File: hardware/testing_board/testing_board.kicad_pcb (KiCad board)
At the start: 2 copper layers, 100.6 x 99.1 mm, 75 parts, among them J1 Conn_01x04, J16 Conn_01x04, J2 Conn_01x04, J3 Conn_01x04, J4 Conn_01x04, J5 Conn_01x04, J6 Conn_01x04, J7 Conn_01x04, J8 Conn_01x04, J9 Conn_01x04, SW1 SW_Push, SW2 SW_Push, SW3 SW_Push, SW4 SW_Push, U1 DS18S20_, U2 DS18S20_, U3 TPIC6595

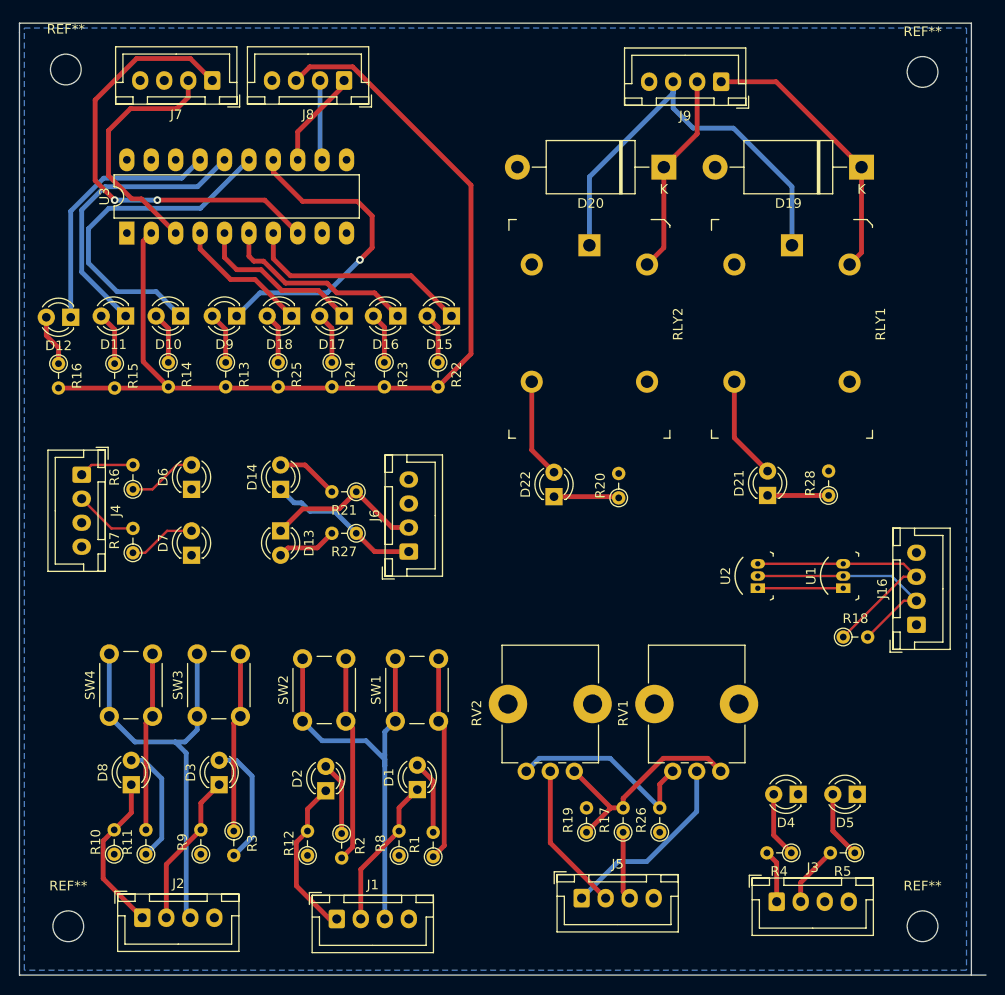
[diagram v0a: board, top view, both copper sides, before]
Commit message: update training bpoard design
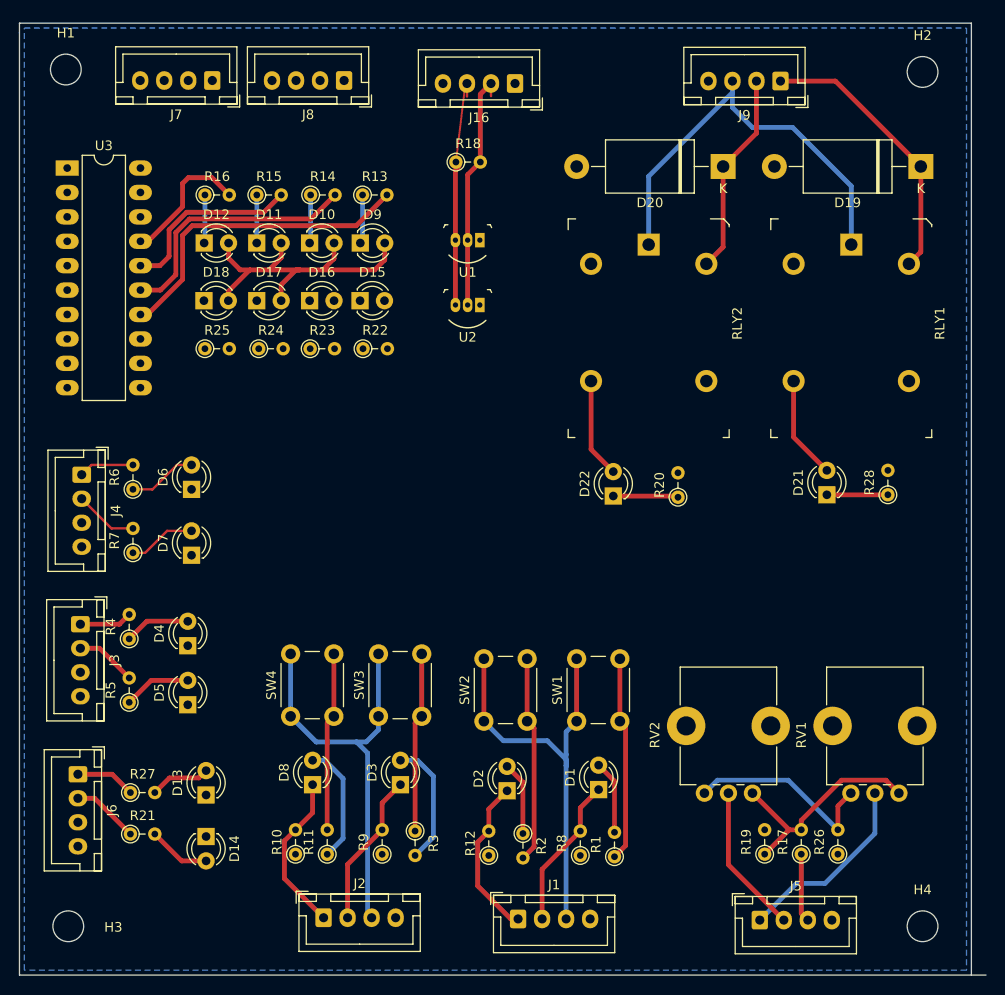
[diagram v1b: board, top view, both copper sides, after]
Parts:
- removed REF** (x4): MountingHole_3.2mm_M3, MountingHole:MountingHole_3.2mm_M3
- added H1: MountingHole, MountingHole:MountingHole_3.2mm_M3_DIN965, F.Cu at (41.7, 25.1)
- added H2: MountingHole, MountingHole:MountingHole_3.2mm_M3_DIN965, F.Cu at (130.8, 25.4)
- added H3: MountingHole, MountingHole:MountingHole_3.2mm_M3_DIN965, F.Cu at (41.9, 114.3)
- added H4: MountingHole, MountingHole:MountingHole_3.2mm_M3_DIN965, F.Cu at (130.8, 114.3)
- moved J3 78.0 mm to (43.2, 82.9), turned to -90 degrees
- moved R5 77.1 mm to (48.2, 91.0), turned to 90 degrees
- moved R4 72.4 mm to (48.2, 84.4), turned to 90 degrees
- moved D5 70.3 mm to (54.3, 91.3), turned to 90 degrees
- moved J16 70.1 mm to (88.4, 26.6), turned to 180 degrees
- moved D4 65.4 mm to (54.3, 85.1), turned to 90 degrees
- moved R18 63.8 mm to (82.2, 34.8)
- moved U1 52.4 mm to (84.7, 42.9), turned to 180 degrees
- moved R21 42.7 mm to (48.4, 104.7), turned to 0 degrees
- moved J6 41.5 mm to (42.9, 98.5), turned to -90 degrees
- moved U2 41.3 mm to (84.7, 49.6), turned to 180 degrees
- moved D14 36.9 mm to (56.2, 105.0), turned to -90 degrees
- moved R27 35.8 mm to (48.4, 100.4), turned to 0 degrees
- moved D13 28.6 mm to (56.2, 100.6), turned to 90 degrees
- moved R16 23.2 mm to (56.1, 38.2), turned to 0 degrees
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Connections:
- D10 pad 1: Net-(D10-Pad1) -> Net-(R14-Pad1)
- D10 pad 2: Net-(D10-Pad2) -> +5V
- D11 pad 2: Net-(D11-Pad2) -> +5V
- D12 pad 1: Net-(D12-Pad1) -> Net-(R16-Pad1)
- D12 pad 2: Net-(D12-Pad2) -> +5V
- D13 pad 1: Net-(D13-Pad1) -> GND
- D14 pad 1: Net-(D14-Pad1) -> GND
- D15 pad 2: Net-(D15-Pad2) -> +5V
- D16 pad 2: Net-(D16-Pad2) -> +5V
- D17 pad 2: Net-(D17-Pad2) -> +5V
- D18 pad 1: Net-(D18-Pad1) -> Net-(R25-Pad1)
- D18 pad 2: Net-(D18-Pad2) -> +5V
- D9 pad 2: Net-(D9-Pad2) -> +5V
- J16 pad 1: Net-(J16-Pad1) -> unconnected-(J16-Pad1)
- J3 pad 3: Net-(J3-Pad3) -> +5V
- J4 pad 3: Net-(J4-Pad3) -> +5V
- J6 pad 1: Net-(D14-Pad1) -> Net-(J6-Pad1)
- J6 pad 2: Net-(D13-Pad1) -> Net-(J6-Pad2)
- R13 pad 1: Net-(D9-Pad2) -> Net-(D9-Pad1)
- R13 pad 2: +5V -> Net-(U3-Pad14)
- R14 pad 1: Net-(D10-Pad2) -> Net-(R14-Pad1)
- R14 pad 2: +5V -> Net-(U3-Pad15)
- R15 pad 1: Net-(D11-Pad2) -> Net-(D11-Pad1)
- R15 pad 2: +5V -> Net-(U3-Pad16)
- R16 pad 1: Net-(D12-Pad2) -> Net-(R16-Pad1)
- R16 pad 2: +5V -> Net-(U3-Pad17)
- R21 pad 1: Net-(D13-Pad1) -> Net-(J6-Pad2)
- R22 pad 1: Net-(D15-Pad2) -> Net-(D15-Pad1)
- R22 pad 2: +5V -> Net-(U3-Pad7)
- R23 pad 1: Net-(D16-Pad2) -> Net-(D16-Pad1)
- R23 pad 2: +5V -> Net-(U3-Pad6)
- R24 pad 1: Net-(D17-Pad2) -> Net-(D17-Pad1)
- R24 pad 2: +5V -> Net-(R24-Pad2)
- R25 pad 1: Net-(D18-Pad2) -> Net-(R25-Pad1)
- R25 pad 2: +5V -> Net-(U3-Pad4)
- R27 pad 1: Net-(D14-Pad1) -> Net-(J6-Pad1)
- RLY1 pad 4: Net-(RLY1-Pad4) -> unconnected-(RLY1-Pad4)
- RLY2 pad 4: Net-(RLY2-Pad4) -> unconnected-(RLY2-Pad4)
- U3 pad 14: Net-(D9-Pad1) -> Net-(U3-Pad14)
- U3 pad 15: Net-(D10-Pad1) -> Net-(U3-Pad15)
- U3 pad 16: Net-(D11-Pad1) -> Net-(U3-Pad16)
- U3 pad 17: Net-(D12-Pad1) -> Net-(U3-Pad17)
- U3 pad 18: Net-(U3-Pad18) -> unconnected-(U3-Pad18)
- U3 pad 4: Net-(D18-Pad1) -> Net-(U3-Pad4)
- U3 pad 5: Net-(D17-Pad1) -> Net-(R24-Pad2)
- U3 pad 6: Net-(D16-Pad1) -> Net-(U3-Pad6)
- U3 pad 7: Net-(D15-Pad1) -> Net-(U3-Pad7)
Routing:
- net +5V: track 272.0 -> 192.4 mm
- net Net-(J7-Pad1): track 46.7 -> 0.00 mm, vias 2 -> 0
- net Net-(D10-Pad1): track 35.1 -> 0.00 mm
- net Net-(U3-Pad14): track 0.00 -> 33.5 mm
- net Net-(D9-Pad1): track 33.8 -> 5.10 mm, vias 1 -> 0
- net Net-(U3-Pad15): track 0.00 -> 26.9 mm
- net Net-(D12-Pad1): track 26.7 -> 0.00 mm
- net Net-(J7-Pad2): track 25.6 -> 0.00 mm
- net Net-(D11-Pad1): track 30.0 -> 5.00 mm
- net Net-(D15-Pad1): track 23.7 -> 0.00 mm
- net Net-(D16-Pad1): track 20.5 -> 0.00 mm
- net Net-(U3-Pad16): track 0.00 -> 19.3 mm
- net Net-(D17-Pad1): track 17.5 -> 0.00 mm
- net Net-(D13-Pad1): track 16.6 -> 0.00 mm
- net Net-(D14-Pad1): track 16.0 -> 0.00 mm
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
